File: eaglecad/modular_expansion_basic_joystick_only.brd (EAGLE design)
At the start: 55.3 x 74.6 mm, 31 parts, among them IC10 74ALS00N, IC11 74ALS00N, IC4 74ALS30N, IC6 74LS00N, IC7 74LS244N, IC8 7805TV, J1 JOY1, J3 POWERJACK

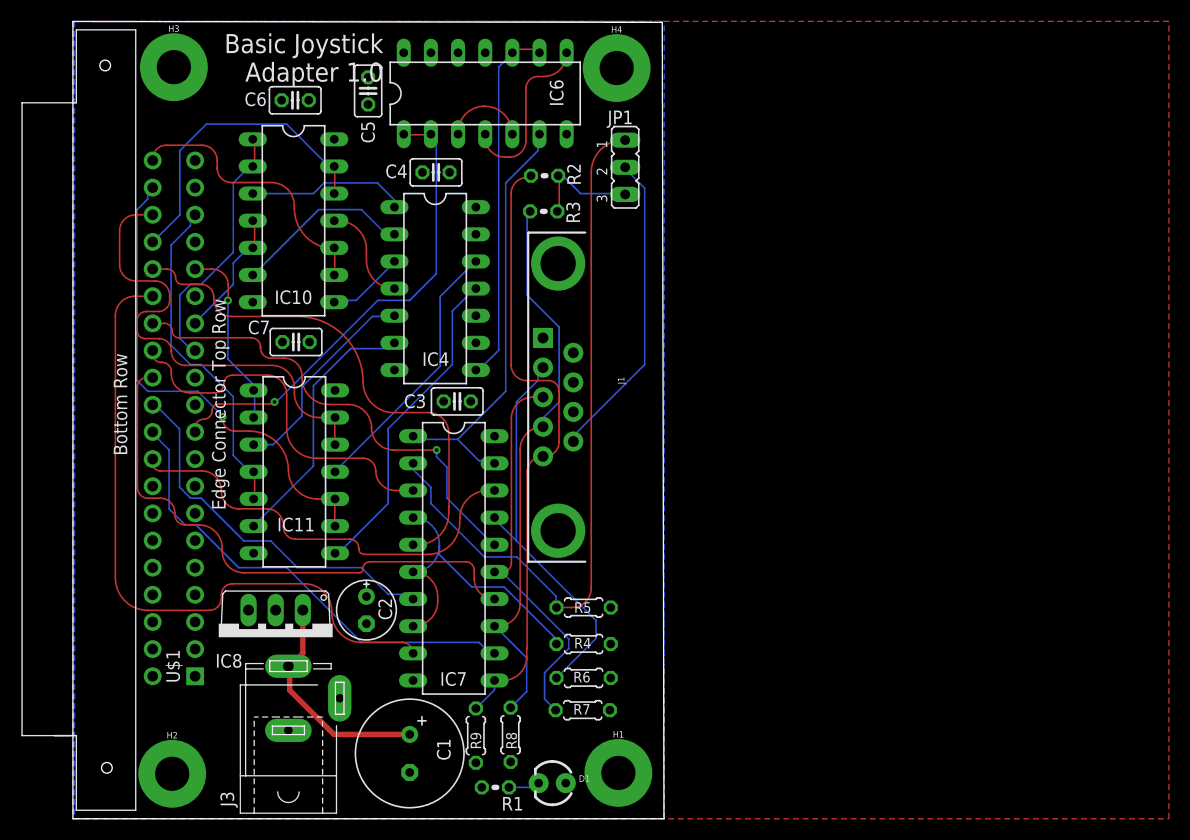
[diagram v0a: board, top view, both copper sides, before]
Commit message: various fixes
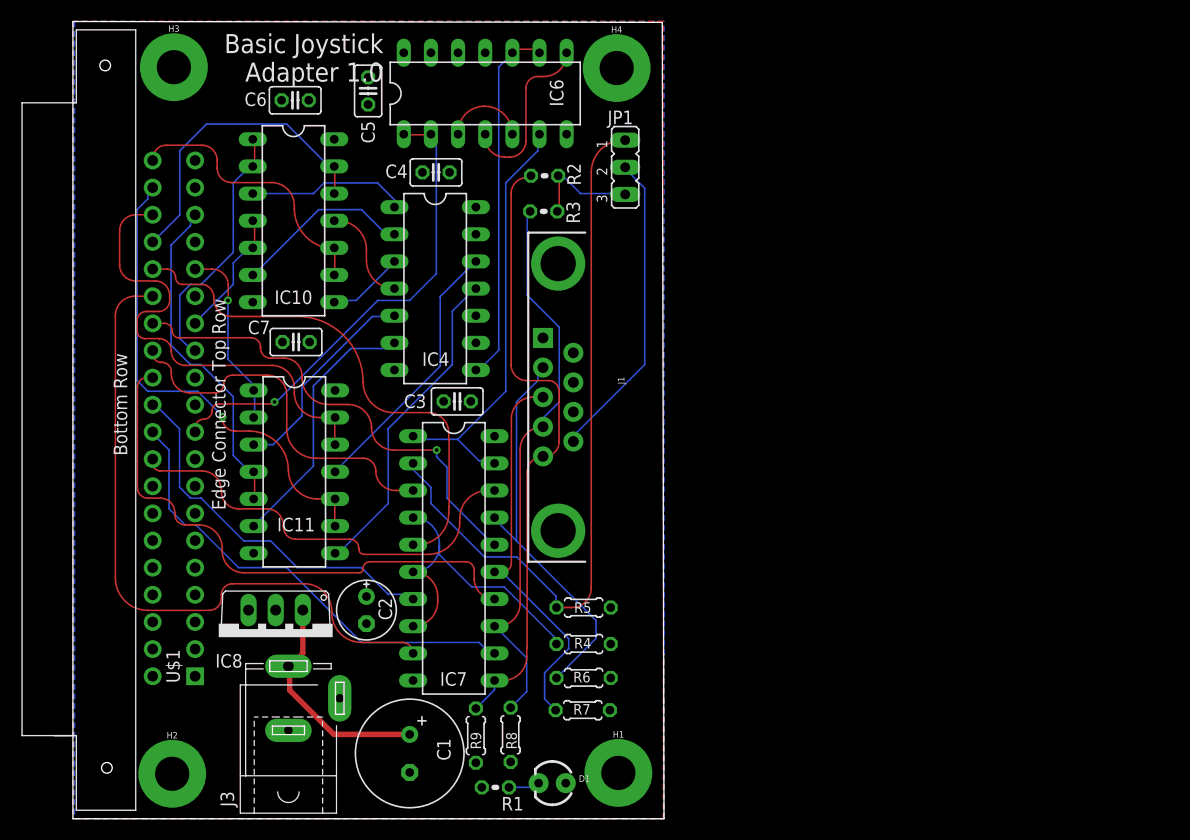
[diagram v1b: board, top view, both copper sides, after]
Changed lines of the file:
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@@
 <polygon width="0.1524" layer="1">
 <vertex x="0" y="0"/>
-<vertex x="102.5525" y="0"/>
-<vertex x="102.5525" y="74.6125"/>
+<vertex x="55.245" y="0"/>
+<vertex x="55.245" y="74.6125"/>
 <vertex x="0" y="74.6125"/>
 </polygon>
